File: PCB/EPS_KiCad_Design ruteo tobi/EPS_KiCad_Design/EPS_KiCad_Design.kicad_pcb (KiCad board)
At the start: 4 copper layers, 90 x 90.2 mm, 133 parts, among them IC1 INA226AIDGST, IC10 TPS2553QDBVRQ1, IC11 INA226AIDGST, IC2 TPS2553QDBVRQ1, IC3 INA226AIDGST, IC4 TPS2553QDBVRQ1, IC5 AP63205WU-7, IC6 STM32L433CBT7, IC7 LT3652IMSE#PBF, IC8 INA226AIDGST, IC9 TPS25921ADR, J1 Conn_02x20_Counter_Clockwise, J10 Conn_01x04, J2 FTSH-107-01-L-D-K, J3 Conn_01x04, J4 Conn_01x04, J5 Conn_01x04, J7 501568-0207, J8 Conn_01x04, J9 Conn_01x04, Y1 ABS07-LR-32.768KHZ-6-1-T, Y2 ABM3-8.000MHZ-D2Y-T

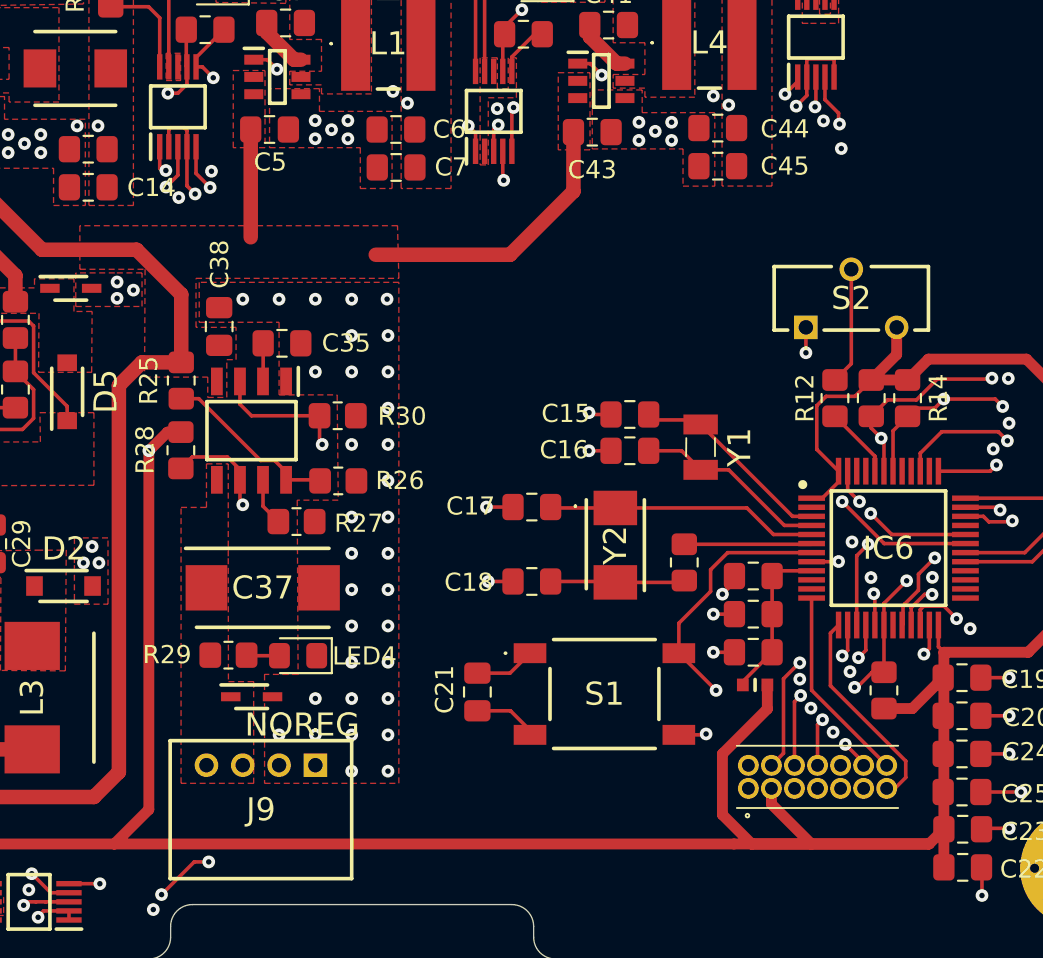
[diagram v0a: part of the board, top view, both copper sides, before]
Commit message: Cambios menores
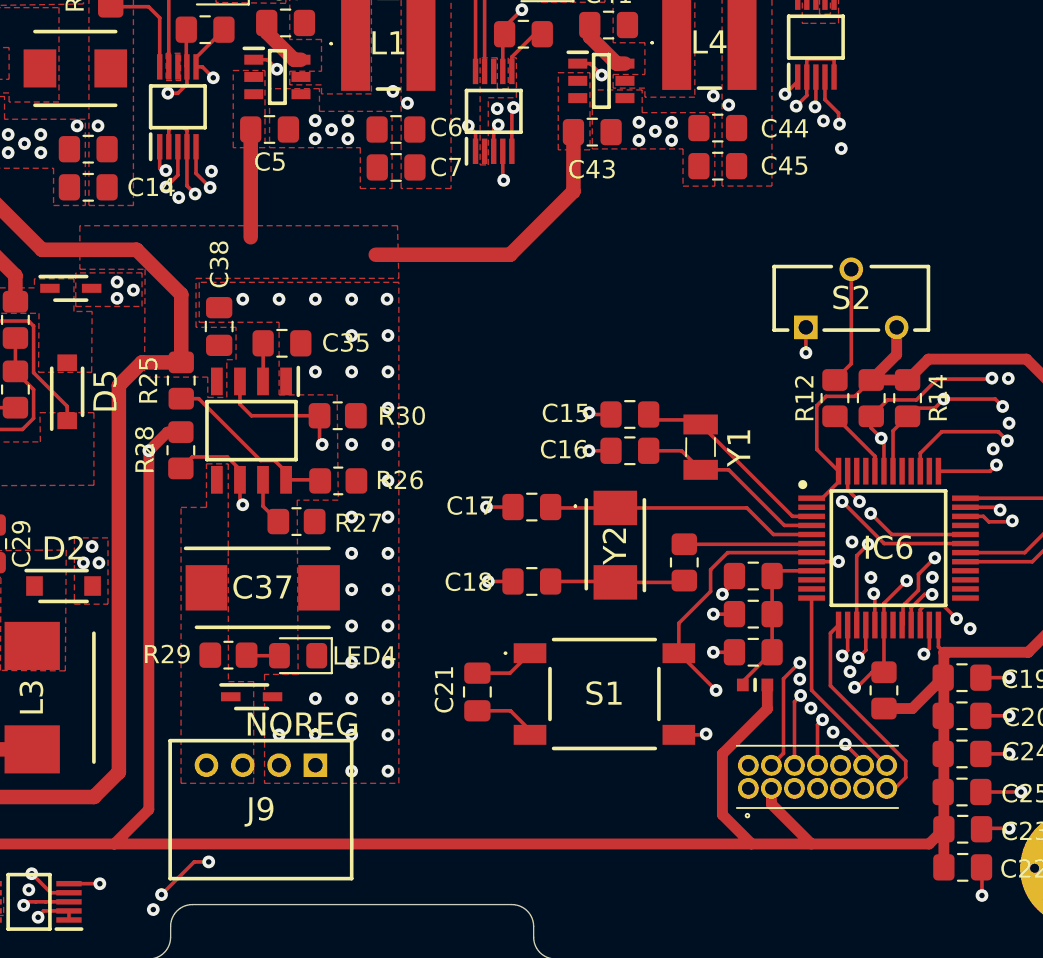
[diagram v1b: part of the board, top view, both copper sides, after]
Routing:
- net 3V3_1: track 230.3 -> 220.6 mm
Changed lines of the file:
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@@
 		(tags "capacitor handsolder")
 		(property "Reference" "C6"
-			(at -2.94 0.01 0)
+			(at -2.7875 0.1 0)
 			(layer "F.SilkS")
 			(effects
@@
 		(sheetname "/MCU/")
 		(sheetfile "MCU.kicad_sch")
+		(clearance 0.12)
 		(attr through_hole)
 		(fp_line
@@
 		(tags "capacitor handsolder")
 		(property "Reference" "C7"
-			(at -3.0325 0.02 0)
+			(at -2.7775 -0.01 0)
 			(layer "F.SilkS")
 			(effects
@@
 	)
 	(segment
-		(start 168.1 133.5)
-		(end 168.1 134.3625)
+		(start 167 136.55)
+		(end 167 136.5625)
 		(width 0.6)
 		(layer "F.Cu")
@@
 	)
 	(segment
-		(start 166.0375 136.5625)
-		(end 167.0125 136.5625)
+		(start 168.1 133.5)
+		(end 168.1 134.3625)
 		(width 0.6)
 		(layer "F.Cu")
@@
 	)
 	(segment
-		(start 133.8 134.6625)
-		(end 133.8 114.9)
+		(start 167.875 127.8)
+		(end 167.875 129.125)
 		(width 0.6)
 		(layer "F.Cu")
@@
 	)
 	(segment
-		(start 166.0375 136.5625)
-		(end 131.9 136.5625)
+		(start 133.8 134.6625)
+		(end 133.8 114.9)
 		(width 0.6)
 		(layer "F.Cu")
@@
 	)
 	(segment
-		(start 170.3 136.5625)
-		(end 176.7875 136.5625)
-		(width 0.6)
-		(layer "F.Cu")
-		(net 15)
-	)
-	(segment
 		(start 134.83 113.87)
 		(end 135.565 113.87)
@@
 	)
 	(segment
-		(start 167.0125 136.5625)
-		(end 176.7875 136.5625)
-		(width 0.6)
-		(layer "F.Cu")
-		(net 15)
-	)
-	(segment
-		(start 167.875 129.125)
-		(end 165.4 131.6)
-		(width 0.6)
-		(layer "F.Cu")
-		(net 15)
-	)
-	(segment
 		(start 173.6 111)
 		(end 175.6 111)
@@
 	)
 	(segment
-		(start 167.875 127.8)
-		(end 167.875 129.125)
+		(start 167.875 129.125)
+		(end 165.4 131.6)
 		(width 0.6)
 		(layer "F.Cu")
@@
 	)
 	(segment
-		(start 167.0125 136.5625)
-		(end 170.3 136.5625)
-		(width 0.6)
-		(layer "F.Cu")
-		(net 15)
-	)
-	(segment
 		(start 186.55 121.7)
 		(end 182.25 126)
@@
 	)
 	(segment
+		(start 165.4 131.6)
+		(end 165.4 134.95)
+		(width 0.6)
+		(layer "F.Cu")
+		(net 15)
+	)
+	(segment
 		(start 152.3 87.85)
 		(end 150.35 85.9)
@@
 	)
 	(segment
-		(start 167 136.55)
-		(end 167 136.5625)
-		(width 0.6)
-		(layer "F.Cu")
-		(net 15)
-	)
-	(segment
 		(start 186.55 115)
 		(end 184.038 117.512)
@@
 	)
 	(segment
-		(start 165.4 131.6)
-		(end 165.4 134.95)
-		(width 0.6)
-		(layer "F.Cu")
-		(net 15)
-	)
-	(segment
 		(start 177.3 124.5)
 		(end 177.3 125.7)
@@
 	)
 	(segment
+		(start 131.9 136.5625)
+		(end 176.7875 136.5625)
+		(width 0.6)
+		(layer "F.Cu")
+		(net 15)
+	)
+	(segment
 		(start 150.35 85.9)
 		(end 149.05 85.9)
@@
 	)
 	(segment
-		(start 165.4 134.95)
-		(end 167.0125 136.5625)
-		(width 0.6)
-		(layer "F.Cu")
-		(net 15)
-	)
-	(segment
 		(start 131.9 136.5625)
 		(end 122.7 136.5625)
@@
 		(layer "F.Cu")
 		(net 15)
+	)
+	(segment
+		(start 165.4 134.95)
+		(end 167 136.55)
+		(width 0.6)
+		(layer "F.Cu")
+		(net 15)
